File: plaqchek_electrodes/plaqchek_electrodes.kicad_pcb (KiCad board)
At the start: 2 copper layers, 1 part, among them J1 Conn_01x03

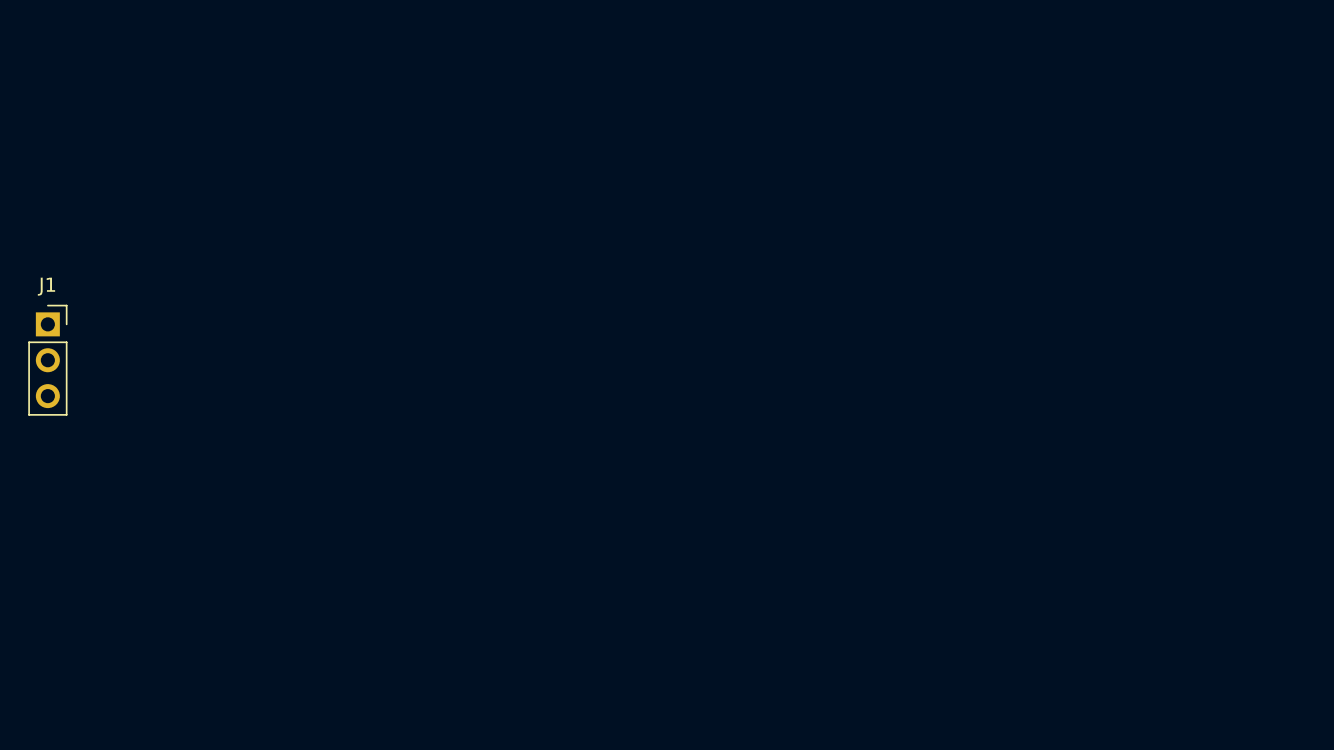
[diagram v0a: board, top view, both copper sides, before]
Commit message: finish all pcbs, generate gerber files
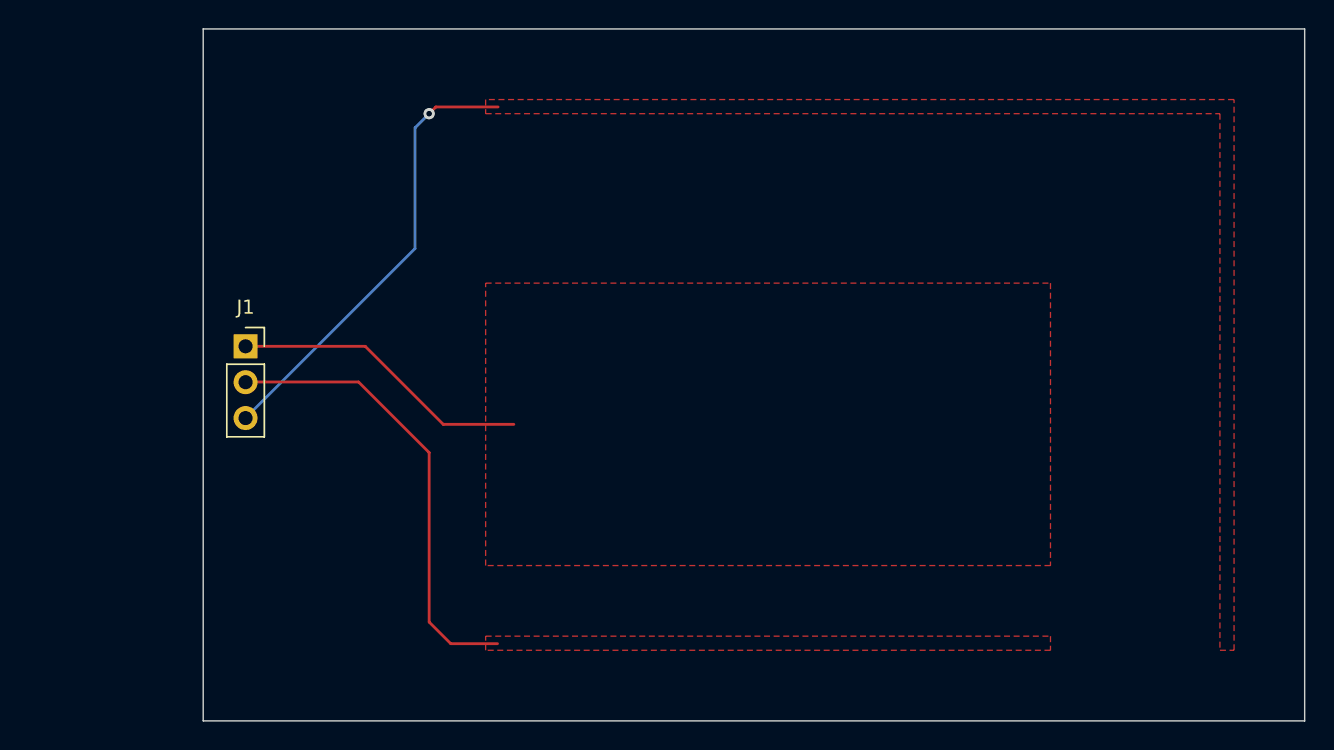
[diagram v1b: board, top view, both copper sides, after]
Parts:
- moved J1 14.1 mm to (144.0, 101.5)
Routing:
- net /REF_ELEC: track 0.00 -> 32.6 mm
- net /COUNTER_ELEC: track 0.00 -> 32.0 mm, vias 0 -> 1
- net /WORKING_ELEC: track 0.00 -> 21.3 mm
- added copper zone on F.Cu, net /COUNTER_ELEC
- added copper zone on F.Cu, net /REF_ELEC
- added copper zone on F.Cu, net /WORKING_ELEC
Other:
- board outline added: 78 x 49 mm
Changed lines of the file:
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@@
       (outputformat 1)
       (mirror false)
-      (drillshape 1)
+      (drillshape 0)
       (scaleselection 1)
-      (outputdirectory "")
+      (outputdirectory "plaqchek_electrodes_gerbers/")
     )
   )
@@
   (net 3 "/COUNTER_ELEC")
   (footprint "Connector_PinSocket_2.54mm:PinSocket_1x03_P2.54mm_Vertical" (layer "F.Cu")
-    (at 130 99.92)
+    (at 144 101.475)
     (descr "Through hole straight socket strip, 1x03, 2.54mm pitch, single row (from Kicad 4.0.7), script generated")
     (tags "Through hole socket strip THT 1x03 2.54mm single row")
@@
     )
   )
+  (gr_rect (start 141 79) (end 219 128)
+    (stroke (width 0.1) (type default)) (fill none) (layer "Edge.Cuts"))
+  (segment (start 158 107) (end 163 107) (width 0.2) (layer "F.Cu") (net 1))
+  (segment (start 152.475 101.475) (end 158 107) (width 0.2) (layer "F.Cu") (net 1))
+  (segment (start 144 101.475) (end 152.475 101.475) (width 0.2) (layer "F.Cu") (net 1))
+  (segment (start 158.532503 122.532503) (end 161.841493 122.532503) (width 0.2) (layer "F.Cu") (net 2))
+  (segment (start 157 109) (end 157 121) (width 0.2) (layer "F.Cu") (net 2))
+  (segment (start 144 104.015) (end 144.015 104) (width 0.2) (layer "F.Cu") (net 2))
+  (segment (start 152 104) (end 157 109) (width 0.2) (layer "F.Cu") (net 2))
+  (segment (start 144.015 104) (end 152 104) (width 0.2) (layer "F.Cu") (net 2))
+  (segment (start 157 121) (end 158.532503 122.532503) (width 0.2) (layer "F.Cu") (net 2))
+  (segment (start 157.476331 84.523669) (end 161.882388 84.523669) (width 0.2) (layer "F.Cu") (net 3))
+  (segment (start 157 85) (end 157.476331 84.523669) (width 0.2) (layer "F.Cu") (net 3))
+  (via (at 157 85) (size 0.8) (drill 0.4) (layers "F.Cu" "B.Cu") (net 3))
+  (segment (start 144 106.555) (end 156 94.555) (width 0.2) (layer "B.Cu") (net 3))
+  (segment (start 156 94.555) (end 156 86) (width 0.2) (layer "B.Cu") (net 3))
+  (segment (start 156 86) (end 157 85) (width 0.2) (layer "B.Cu") (net 3))
+  (zone (net 1) (net_name "/WORKING_ELEC") (layer "F.Cu") (hatch edge 0.5)
+    (priority 1)
+    (connect_pads (clearance 0.5))
+    (min_thickness 0.25) (filled_areas_thickness no)
+    (fill yes (thermal_gap 0.5) (thermal_bridge_width 0.5))
+    (polygon
+      (pts
+        (xy 161 97)
+        (xy 201 97)
+        (xy 201 117)
+        (xy 161 117)
+      )
+    )
+  )
+  (zone (net 2) (net_name "/REF_ELEC") (layer "F.Cu") (hatch edge 0.5)
+    (priority 2)
+    (connect_pads (clearance 0.5))
+    (min_thickness 0.25) (filled_areas_thickness no)
+    (fill yes (thermal_gap 0.5) (thermal_bridge_width 0.5))
+    (polygon
+      (pts
+        (xy 161 122)
+        (xy 201 122)
+        (xy 201 123)
+        (xy 161 123)
+      )
+    )
+  )
+  (zone (net 3) (net_name "/COUNTER_ELEC") (layer "F.Cu") (hatch edge 0.5)
+    (connect_pads (clearance 0.5))
+    (min_thickness 0.25) (filled_areas_thickness no)
+    (fill yes (thermal_gap 0.5) (thermal_bridge_width 0.5))
+    (polygon
+      (pts
+        (xy 161 84)
+        (xy 161 85)
+        (xy 213 85)
+        (xy 213 123)
+        (xy 214 123)
+        (xy 214 84)
+      )
+    )
+  )
+  (zone (net 0) (net_name "") (layer "F.Mask") (hatch edge 0.5)
+    (connect_pads (clearance 0.5))
+    (min_thickness 0.25) (filled_areas_thickness no)
+    (fill yes (thermal_gap 0.5) (thermal_bridge_width 0.5))
+    (polygon
+      (pts
+        (xy 161 122)
+        (xy 201 122)
+        (xy 201 123)
+        (xy 161 123)
+      )
+    )
+  )
+  (zone (net 0) (net_name "") (layer "F.Mask") (hatch edge 0.5)
+    (connect_pads (clearance 0.5))
+    (min_thickness 0.25) (filled_areas_thickness no)
+    (fill yes (thermal_gap 0.5) (thermal_bridge_width 0.5))
+    (polygon
+      (pts
+        (xy 161 97)
+        (xy 201 97)
+        (xy 201 117)
+        (xy 161 117)
+      )
+    )
+  )
+  (zone (net 0) (net_name "") (layer "F.Mask") (hatch edge 0.5)
+    (connect_pads (clearance 0.5))
+    (min_thickness 0.25) (filled_areas_thickness no)
+    (fill yes (thermal_gap 0.5) (thermal_bridge_width 0.5))
+    (polygon
+      (pts
+        (xy 161 84)
+        (xy 161 85)
+        (xy 213 85)
+        (xy 213 123)
+        (xy 214 123)
+        (xy 214 84)
+      )
+    )
+  )
